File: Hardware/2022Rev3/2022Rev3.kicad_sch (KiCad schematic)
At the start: 2 parts

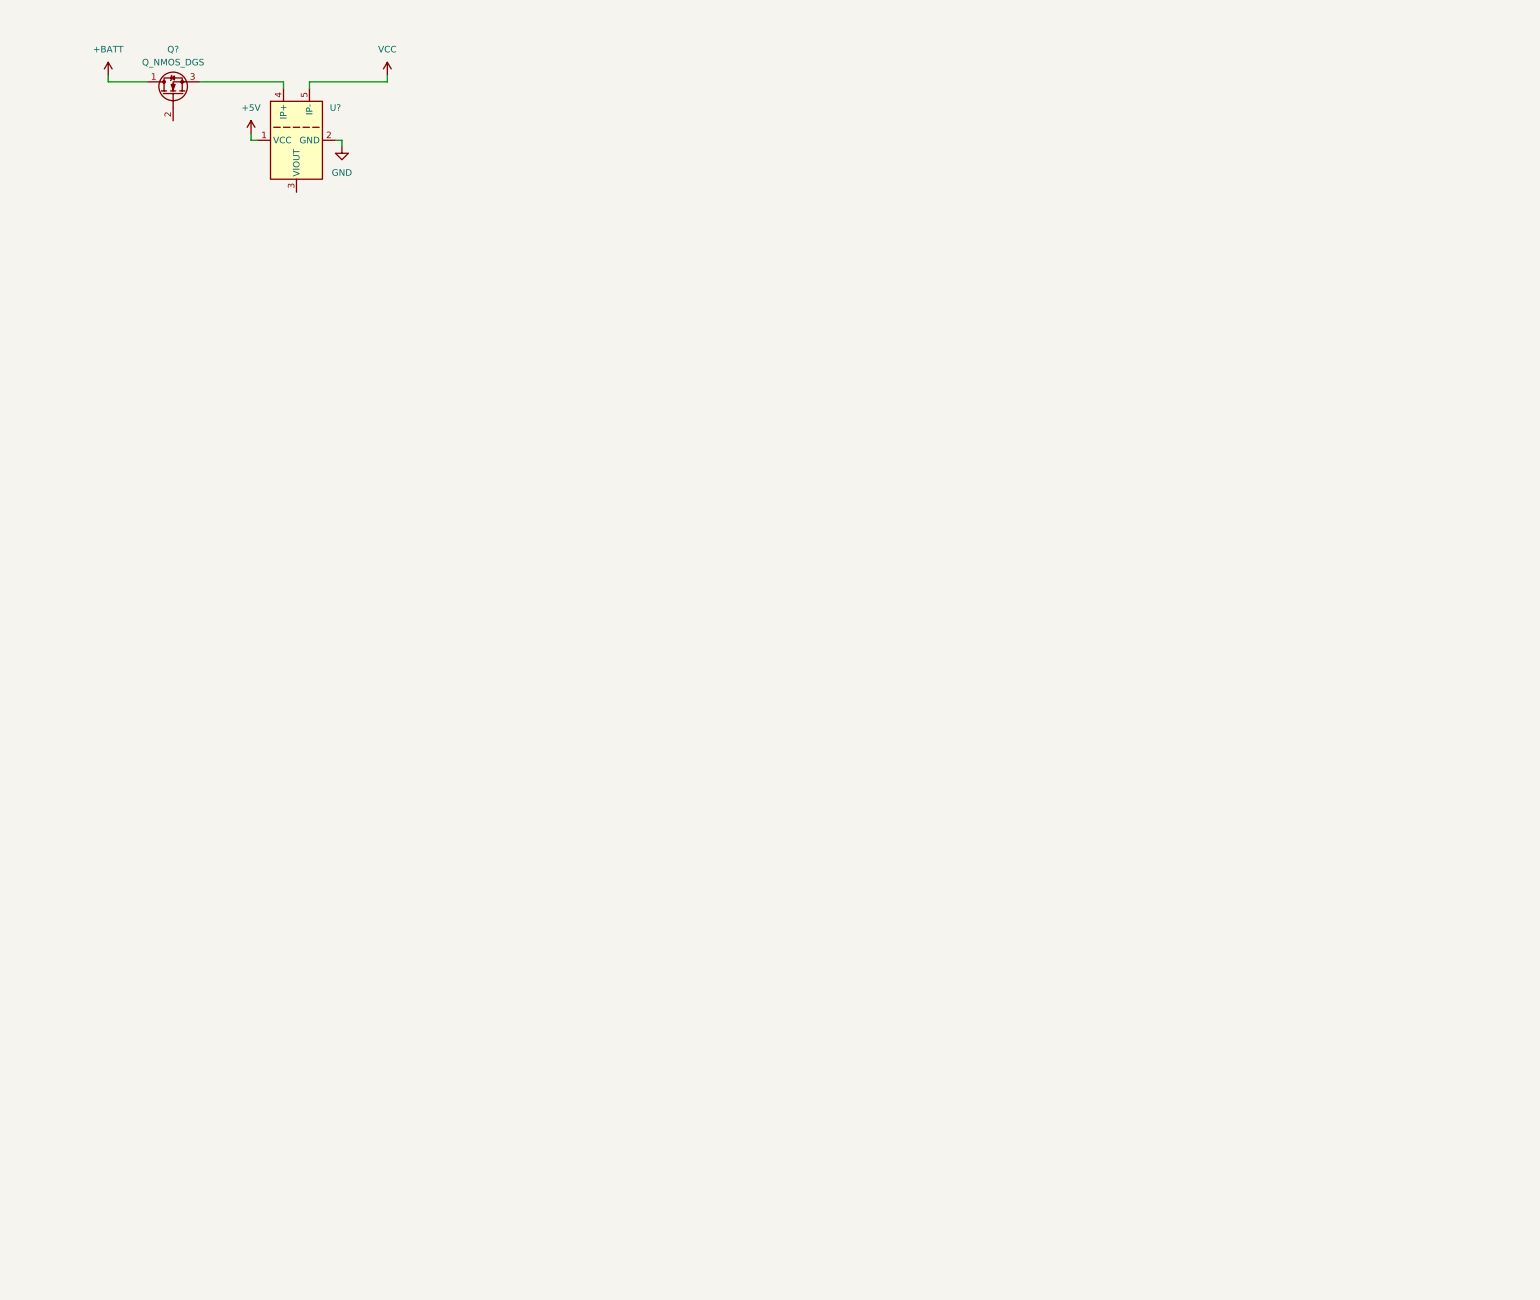
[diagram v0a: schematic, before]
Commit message: circuit addition
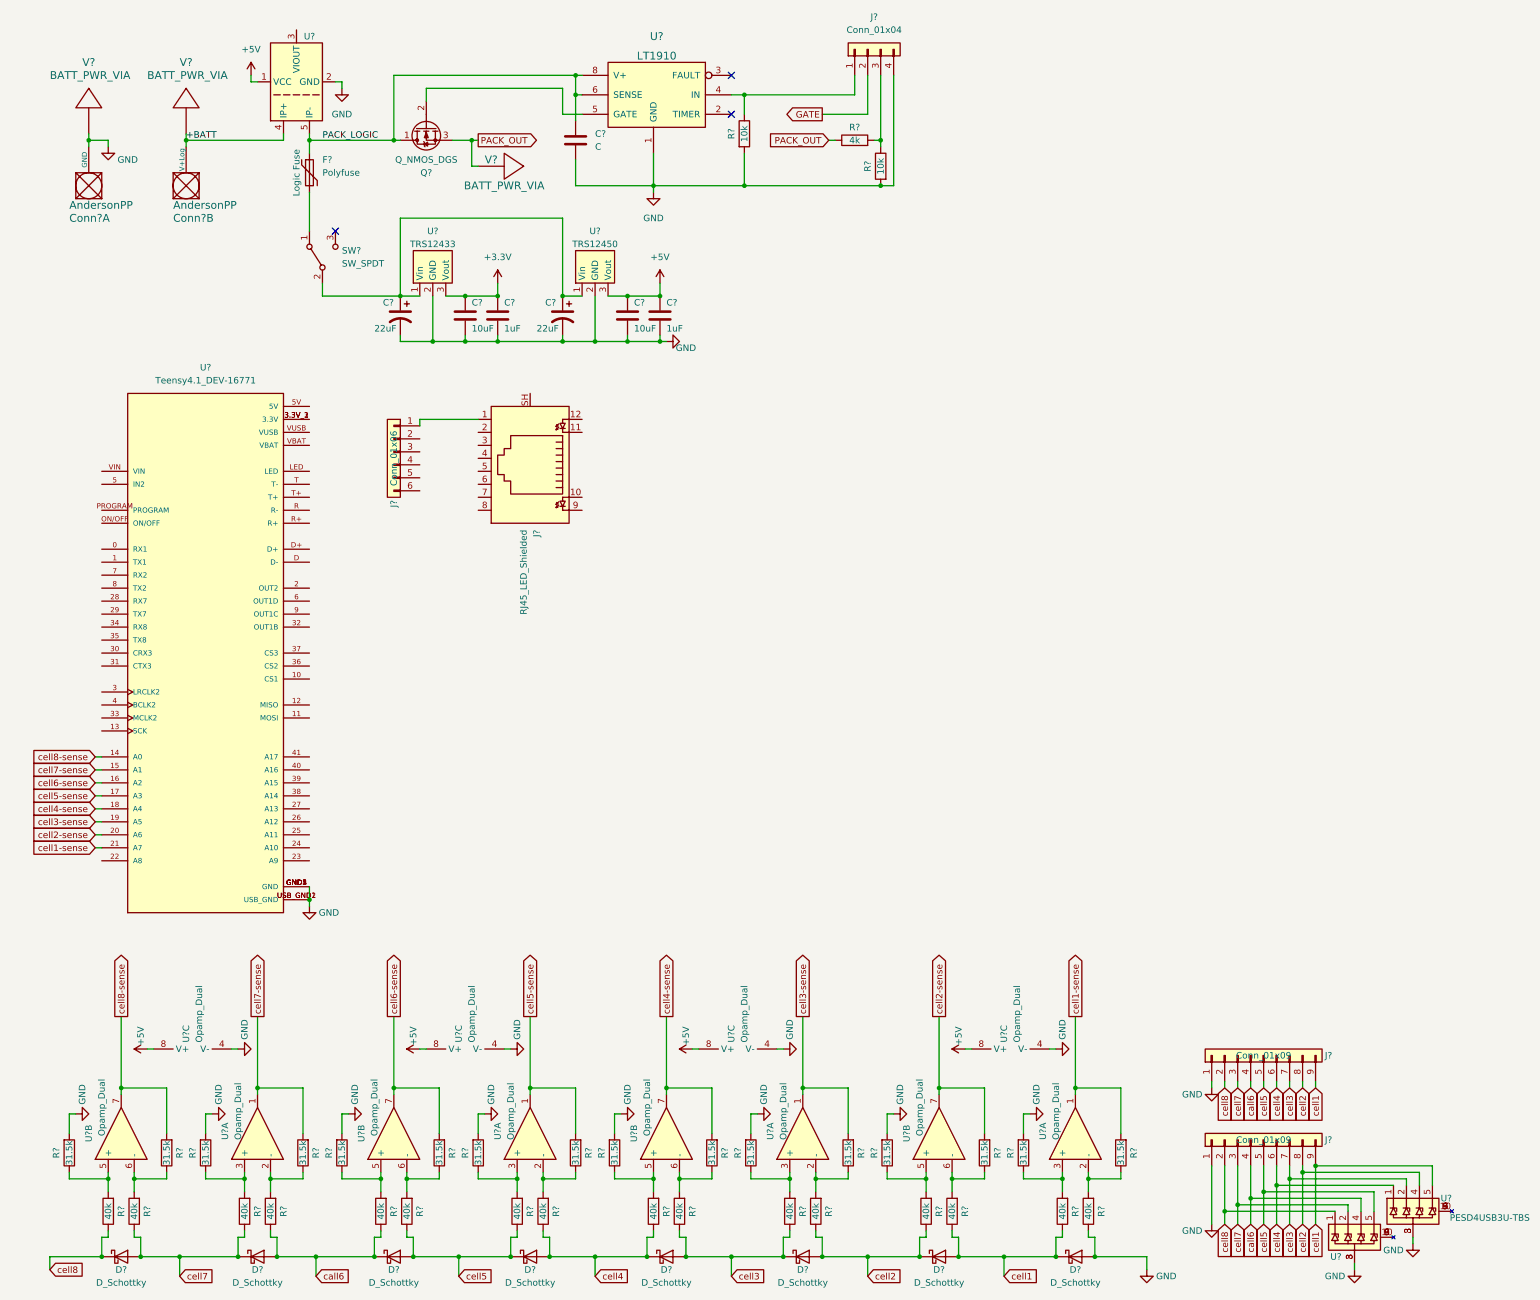
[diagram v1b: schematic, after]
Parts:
- added C? (x2): 10uF, symbol Device:C
- added C? (x2): 22uF, symbol Device:C_Polarized_US
- added C? (x2): 1uF, symbol Device:C
- added C?: C, symbol Device:C
- added Conn? (x2): AndersonPP, symbol MRDT_Connectors:AndersonPP
- added D? (x8): D_Schottky, symbol Device:D_Schottky
- added F?: Polyfuse, symbol Device:Polyfuse
- added J? (x2): Conn_01x09, symbol Connector_Generic:Conn_01x09
- added J?: Conn_01x06, symbol Connector_Generic:Conn_01x06
- added J?: RJ45_LED_Shielded, symbol Connector:RJ45_LED_Shielded
- added J?: Conn_01x04, symbol Connector_Generic:Conn_01x04
- added R? (x16): 31.5k, symbol Device:R
- added R? (x16): 40k, symbol Device:R
- added R?: 4k, symbol Device:R
- added R? (x2): 10k, symbol Device:R
- added SW?: SW_SPDT, symbol Switch:SW_SPDT
- added U?: Teensy4.1_DEV-16771, MODULE_DEV-16771, symbol MRDT_Shields:Teensy4.1_DEV-16771
- added U? (x12): Opamp_Dual, symbol Device:Opamp_Dual
- added U? (x2): PESD4USB3U-TBS, symbol BMSRev3:PESD4USB3U-TBS
- added U?: LT1910, symbol MRDT_ICs:LT1910
- added U?: TRS12450, symbol BMSRev3:TRS12433
- added U?: TRS12433, symbol BMSRev3:TRS12433
- added V? (x3): BATT_PWR_VIA, symbol MRDT_Drill_Holes:BATT_PWR_VIA
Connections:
- net +5V: now also C?.1, C?.1, U?.3 (Vout), U?.8 (V+), U?.8 (V+), U?.8 (V+), U?.8 (V+)
- net +BATT: now also U?.4 (IP+), Conn?.2 (V+Log), V?.1; no longer Q?.1 (D)
- net GND: now also C?.2, C?.2, C?.2, C?.2, C?.2, C?.2, C?.2, Conn?.1 (GND), D?.2 (A), J?.1 (Pin_1), J?.1 (Pin_1), J?.4 (Pin_4), R?.1, R?.2, R?.2, R?.2, R?.2, R?.2, R?.2, R?.2, R?.2, R?.2, R?.2, U?.1 (GND), U?.2 (GND), U?.2 (GND), U?.3, U?.3, U?.4 (V-), U?.4 (V-), U?.4 (V-), U?.4 (V-), U?.8, U?.8, U?.GND1 (GND), U?.GND2 (GND), U?.GND3 (GND), U?.GND4 (GND), U?.GND5 (GND), U?.USB_GND1 (USB_GND), U?.USB_GND2 (USB_GND), V?.1
- net PACK_OUT: now reaches Q?.3 (S)
- net PACK_OUT: now also R?.1, V?.1; no longer U?.4 (IP+)
- net at Q?.2 (G): now also U?.5 (GATE)
- net VCC renamed PACK_LOGIC
- net PACK_LOGIC: now also Q?.1 (D), C?.1, F?.1, U?.6 (SENSE), U?.8 (V+)
- new net: U?.3.3V_1 (3.3V), U?.3.3V_2 (3.3V), U?.3.3V_3 (3.3V)
- new net: R?.1, R?.2, U?.6 (-) (x4)
- new net: R?.1, R?.2, U?.2 (-) (x4)
- new net: F?.2, SW?.1 (A)
- new net: C?.1, C?.1, SW?.2 (B), U?.1 (Vin), U?.1 (Vin)
- new net: J?.1, J?.1 (Pin_1)
- new net: R?.1, R?.2, U?.5 (+) (x4)
- new net: R?.1, R?.2, U?.3 (+) (x4)
- new net: U?.10, U?.6, U?.7, U?.9 (x2)
- new net: J?.3 (Pin_3), R?.1, R?.2
- new net: J?.1 (Pin_1), R?.1, U?.4 (IN)
- new net +3V3: C?.1, C?.1, U?.3 (Vout)
- new net GATE: J?.2 (Pin_2)
- new net call6: D?.1 (K), D?.2 (A), J?.4 (Pin_4), J?.4 (Pin_4), R?.1, R?.1, U?.4
- new net cell1: D?.1 (K), D?.2 (A), J?.9 (Pin_9), J?.9 (Pin_9), R?.1, R?.1, U?.5
- new net cell1-sense: R?.2, U?.1, U?.21 (A7)
- new net cell2: D?.1 (K), D?.2 (A), J?.8 (Pin_8), J?.8 (Pin_8), R?.1, R?.1, U?.4
- new net cell2-sense: R?.2, U?.20 (A6), U?.7
- new net cell3: D?.1 (K), D?.2 (A), J?.7 (Pin_7), J?.7 (Pin_7), R?.1, R?.1, U?.2
- new net cell3-sense: R?.2, U?.1, U?.19 (A5)
- new net cell4: D?.1 (K), D?.2 (A), J?.6 (Pin_6), J?.6 (Pin_6), R?.1, R?.1, U?.1
- new net cell4-sense: R?.2, U?.18 (A4), U?.7
- new net cell5: D?.1 (K), D?.2 (A), J?.5 (Pin_5), J?.5 (Pin_5), R?.1, R?.1, U?.5
- new net cell5-sense: R?.2, U?.1, U?.17 (A3)
- new net cell6-sense: R?.2, U?.16 (A2), U?.7
- new net cell7: D?.1 (K), D?.2 (A), J?.3 (Pin_3), J?.3 (Pin_3), R?.1, R?.1, U?.2
- new net cell7-sense: R?.2, U?.1, U?.15 (A1)
- new net cell8: D?.1 (K), J?.2 (Pin_2), J?.2 (Pin_2), R?.1, U?.1
- new net cell8-sense: R?.2, U?.14 (A0), U?.7
- no-connect marks 0 -> 3
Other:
- company: (none) -> Mars Rover Design Team
- title: (none) -> Battery Management System
- moved on the sheet: Q?, U?
